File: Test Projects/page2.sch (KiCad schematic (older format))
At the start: 20 parts, among them P3 COLS0, P32 PIN8, P33 SIO2, P34 ~HOLD~/SIO3, P35 PIN37, P37 PIN31, P4 COLS1, U3 Teensy_3.2, U32 SPI_MEMORY_SOIC8, U6 SF-MicroSD-12term, U7 SF-74HC595, U8 SF-74HC595

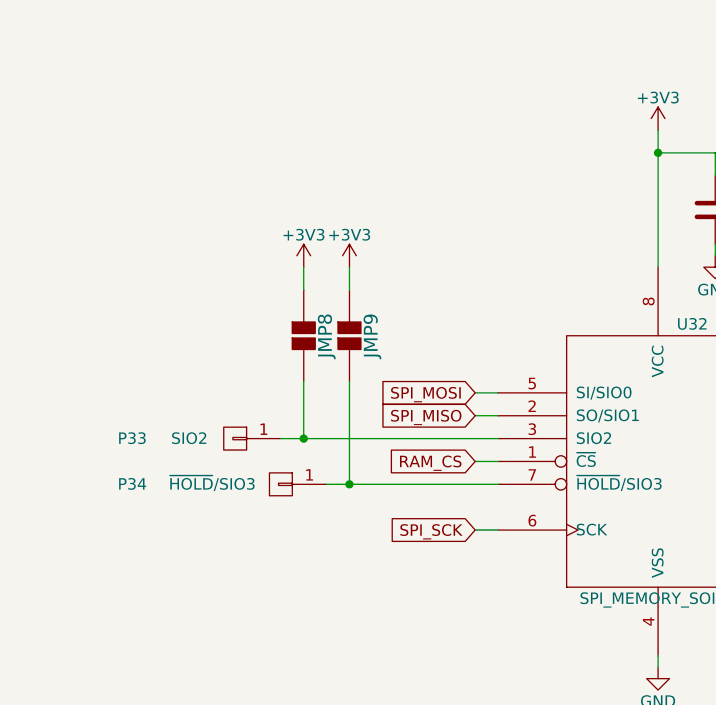
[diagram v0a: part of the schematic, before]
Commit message: layout
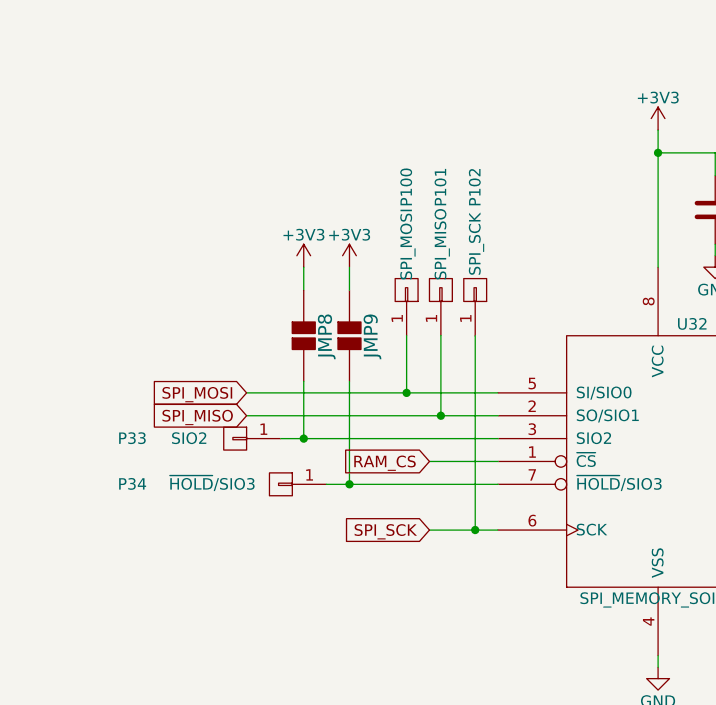
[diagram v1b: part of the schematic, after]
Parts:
- added P100: SPI_MOSI, SparkFun-Footprints:TestHole, symbol CONN_01X01
- added P101: SPI_MISO, SparkFun-Footprints:TestHole, symbol CONN_01X01
- added P102: SPI_SCK, SparkFun-Footprints:TestHole, symbol CONN_01X01
- P32, P33, P34, P35, P37: footprint SparkFun-Footprints:Single_PTH -> SparkFun-Footprints:TestHole
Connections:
- net SPI_MISO: now also P101.1 (P1)
- net SPI_MOSI: now also P100.1 (P1)
- net SPI_SCK: now also P102.1 (P1)
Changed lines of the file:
@@
 LIBS:SparkFun-Mounting
 LIBS:SparkFun-Opto
+LIBS:SparkFun-Connectors
 LIBS:Teensy_test_layout-cache
 EELAYER 25 0
@@
 SPI_MOSI
 $Comp
-L +3V3 #PWR019
+L +3V3 #PWR020
 U 1 1 568C434E
 P 8350 1550
-F 0 "#PWR019" H 8350 1400 50  0001 C CNN
+F 0 "#PWR020" H 8350 1400 50  0001 C CNN
 F 1 "+3V3" H 8350 1690 50  0000 C CNN
 F 2 "" H 8350 1550 50  0000 C CNN
@@
 $EndComp
 $Comp
-L +3V3 #PWR020
+L +3V3 #PWR021
 U 1 1 568C4354
 P 8150 1550
-F 0 "#PWR020" H 8150 1400 50  0001 C CNN
+F 0 "#PWR021" H 8150 1400 50  0001 C CNN
 F 1 "+3V3" H 8150 1690 50  0000 C CNN
 F 2 "" H 8150 1550 50  0000 C CNN
@@
 F 0 "P32" H 5850 2650 50  0000 C CNN
 F 1 "PIN8" H 5650 2650 50  0000 C CNN
-F 2 "SparkFun-Footprints:Single_PTH" H 5500 2650 50  0001 C CNN
+F 2 "SparkFun-Footprints:TestHole" H 5500 2650 50  0001 C CNN
 F 3 "" H 5500 2650 50  0000 C CNN
 	1    5500 2650
@@
 F 0 "P35" H 9200 3150 50  0000 C CNN
 F 1 "PIN37" H 9000 3150 50  0000 C CNN
-F 2 "SparkFun-Footprints:Single_PTH" H 8800 3150 50  0001 C CNN
+F 2 "SparkFun-Footprints:TestHole" H 8800 3150 50  0001 C CNN
 F 3 "" H 8800 3150 50  0000 C CNN
 	1    8800 3150
@@
 $EndComp
 $Comp
-L GND #PWR021
+L GND #PWR022
 U 1 1 56A0F405
 P 3750 1950
-F 0 "#PWR021" H 3750 1700 50  0001 C CNN
+F 0 "#PWR022" H 3750 1700 50  0001 C CNN
 F 1 "GND" H 3750 1800 50  0000 C CNN
 F 2 "" H 3750 1950 50  0000 C CNN
@@
 $EndComp
 $Comp
-L GND #PWR022
+L GND #PWR023
 U 1 1 56A0F6ED
 P 3500 3750
-F 0 "#PWR022" H 3500 3500 50  0001 C CNN
+F 0 "#PWR023" H 3500 3500 50  0001 C CNN
 F 1 "GND" H 3500 3600 50  0000 C CNN
 F 2 "" H 3500 3750 50  0000 C CNN
@@
 $EndComp
 $Comp
-L GND #PWR023
+L GND #PWR024
 U 1 1 56A0FB18
 P 2700 7400
-F 0 "#PWR023" H 2700 7150 50  0001 C CNN
+F 0 "#PWR024" H 2700 7150 50  0001 C CNN
 F 1 "GND" H 2700 7250 50  0000 C CNN
 F 2 "" H 2700 7400 50  0000 C CNN
@@
 $EndComp
 $Comp
-L GND #PWR024
+L GND #PWR025
 U 1 1 56A0FBC8
 P 5200 7400
-F 0 "#PWR024" H 5200 7150 50  0001 C CNN
+F 0 "#PWR025" H 5200 7150 50  0001 C CNN
 F 1 "GND" H 5200 7250 50  0000 C CNN
 F 2 "" H 5200 7400 50  0000 C CNN
@@
 $EndComp
 $Comp
-L +3V3 #PWR025
+L +3V3 #PWR026
 U 1 1 56A0FE25
 P 3500 1400
-F 0 "#PWR025" H 3500 1250 50  0001 C CNN
+F 0 "#PWR026" H 3500 1250 50  0001 C CNN
 F 1 "+3V3" H 3500 1540 50  0000 C CNN
 F 2 "" H 3500 1400 50  0000 C CNN
@@
 $EndComp
 $Comp
-L +3V3 #PWR026
+L +3V3 #PWR027
 U 1 1 56A104A5
 P 2700 6300
-F 0 "#PWR026" H 2700 6150 50  0001 C CNN
+F 0 "#PWR027" H 2700 6150 50  0001 C CNN
 F 1 "+3V3" H 2700 6440 50  0000 C CNN
 F 2 "" H 2700 6300 50  0000 C CNN
@@
 $EndComp
 $Comp
-L +3V3 #PWR027
+L +3V3 #PWR028
 U 1 1 56A105FA
 P 5200 6300
-F 0 "#PWR027" H 5200 6150 50  0001 C CNN
+F 0 "#PWR028" H 5200 6150 50  0001 C CNN
 F 1 "+3V3" H 5200 6440 50  0000 C CNN
 F 2 "" H 5200 6300 50  0000 C CNN
@@
 Connection ~ 5200 6350
 Connection ~ 5200 7350
-Text GLabel 2700 2850 0    50   Input ~ 0
+Text GLabel 2500 2850 0    50   Input ~ 0
 RAM_CS
 Wire Wire Line
-	2800 2850 2700 2850
-Text GLabel 2700 2550 0    50   Input ~ 0
+	2800 2850 2500 2850
+Text GLabel 1700 2550 0    50   Input ~ 0
 SPI_MOSI
-Text GLabel 2700 3150 0    50   Input ~ 0
+Text GLabel 2500 3150 0    50   Input ~ 0
 SPI_SCK
-Text GLabel 2700 2650 0    50   Input ~ 0
+Text GLabel 1700 2650 0    50   Input ~ 0
 SPI_MISO
 $Comp
-L +3V3 #PWR028
+L +3V3 #PWR029
 U 1 1 56A12235
 P 2150 2000
-F 0 "#PWR028" H 2150 1850 50  0001 C CNN
+F 0 "#PWR029" H 2150 1850 50  0001 C CNN
 F 1 "+3V3" H 2150 2140 50  0000 C CNN
 F 2 "" H 2150 2000 50  0000 C CNN
@@
 $EndComp
 $Comp
-L +3V3 #PWR029
+L +3V3 #PWR030
 U 1 1 56A12282
 P 1950 2000
-F 0 "#PWR029" H 1950 1850 50  0001 C CNN
+F 0 "#PWR030" H 1950 1850 50  0001 C CNN
 F 1 "+3V3" H 1950 2140 50  0000 C CNN
 F 2 "" H 1950 2000 50  0000 C CNN
@@
 F 0 "P33" H 2100 2750 50  0000 C CNN
 F 1 "SIO2" H 1850 2750 50  0000 C CNN
-F 2 "SparkFun-Footprints:Single_PTH" H 1650 2750 50  0001 C CNN
+F 2 "SparkFun-Footprints:TestHole" H 1650 2750 50  0001 C CNN
 F 3 "" H 1650 2750 50  0000 C CNN
 	1    1650 2750
@@
 F 0 "P34" H 2500 2950 50  0000 C CNN
 F 1 "~HOLD~/SIO3" H 2150 2950 50  0000 C CNN
-F 2 "SparkFun-Footprints:Single_PTH" H 1850 2950 50  0001 C CNN
+F 2 "SparkFun-Footprints:TestHole" H 1850 2950 50  0001 C CNN
 F 3 "" H 1850 2950 50  0000 C CNN
 	1    1850 2950
@@
 Connection ~ 2150 2950
 Wire Wire Line
-	2700 3150 2800 3150
-Wire Wire Line
-	2700 2650 2800 2650
-Wire Wire Line
-	2700 2550 2800 2550
-$Comp
-L +3V3 #PWR030
+	2500 3150 2800 3150
+Wire Wire Line
+	1700 2650 2800 2650
+Wire Wire Line
+	1700 2550 2800 2550
+$Comp
+L +3V3 #PWR031
 U 1 1 56A16EA5
 P 1200 5150
-F 0 "#PWR030" H 1200 5000 50  0001 C CNN
+F 0 "#PWR031" H 1200 5000 50  0001 C CNN
 F 1 "+3V3" H 1200 5290 50  0000 C CNN
 F 2 "" H 1200 5150 50  0000 C CNN
@@
 $EndComp
 $Comp
-L +3V3 #PWR031
+L +3V3 #PWR032
 U 1 1 56A16EFE
 P 3750 5100
-F 0 "#PWR031" H 3750 4950 50  0001 C CNN
+F 0 "#PWR032" H 3750 4950 50  0001 C CNN
 F 1 "+3V3" H 3750 5240 50  0000 C CNN
 F 2 "" H 3750 5100 50  0000 C CNN
@@
 F 0 "P37" H 9200 3850 50  0000 C CNN
 F 1 "PIN31" H 9000 3850 50  0000 C CNN
-F 2 "SparkFun-Footprints:Single_PTH" H 8800 3850 50  0001 C CNN
+F 2 "SparkFun-Footprints:TestHole" H 8800 3850 50  0001 C CNN
 F 3 "" H 8800 3850 50  0000 C CNN
 	1    8800 3850
@@
 Text GLabel 9000 2150 0    50   Input ~ 0
 D
+$Comp
+L CONN_01X01 P100
+U 1 1 56AFECCB
+P 2400 2100
+F 0 "P100" H 2850 2100 50  0000 C CNN
+F 1 "SPI_MOSI" H 2600 2100 50  0000 C CNN
+F 2 "SparkFun-Footprints:TestHole" H 2400 2100 50  0001 C CNN
+F 3 "" H 2400 2100 50  0000 C CNN
+	1    2400 2100
+	0    1    -1   0
+$EndComp
+$Comp
+L CONN_01X01 P101
+U 1 1 56AFED56
+P 2550 2100
+F 0 "P101" H 3000 2100 50  0000 C CNN
+F 1 "SPI_MISO" H 2750 2100 50  0000 C CNN
+F 2 "SparkFun-Footprints:TestHole" H 2550 2100 50  0001 C CNN
+F 3 "" H 2550 2100 50  0000 C CNN
+	1    2550 2100
+	0    1    -1   0
+$EndComp
+$Comp
+L CONN_01X01 P102
+U 1 1 56AFEDB8
+P 2700 2100
+F 0 "P102" H 3150 2100 50  0000 C CNN
+F 1 "SPI_SCK" H 2900 2100 50  0000 C CNN
+F 2 "SparkFun-Footprints:TestHole" H 2700 2100 50  0001 C CNN
+F 3 "" H 2700 2100 50  0000 C CNN
+	1    2700 2100
+	0    1    -1   0
+$EndComp
+Wire Wire Line
+	2400 2300 2400 2550
+Connection ~ 2400 2550
+Wire Wire Line
+	2550 2300 2550 2650
+Connection ~ 2550 2650
+Wire Wire Line
+	2700 2300 2700 3150
+Connection ~ 2700 3150
 $EndSCHEMATC
